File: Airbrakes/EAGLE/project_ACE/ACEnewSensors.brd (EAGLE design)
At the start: 100.3 x 62.2 mm, 21 parts, among them J3 PTH

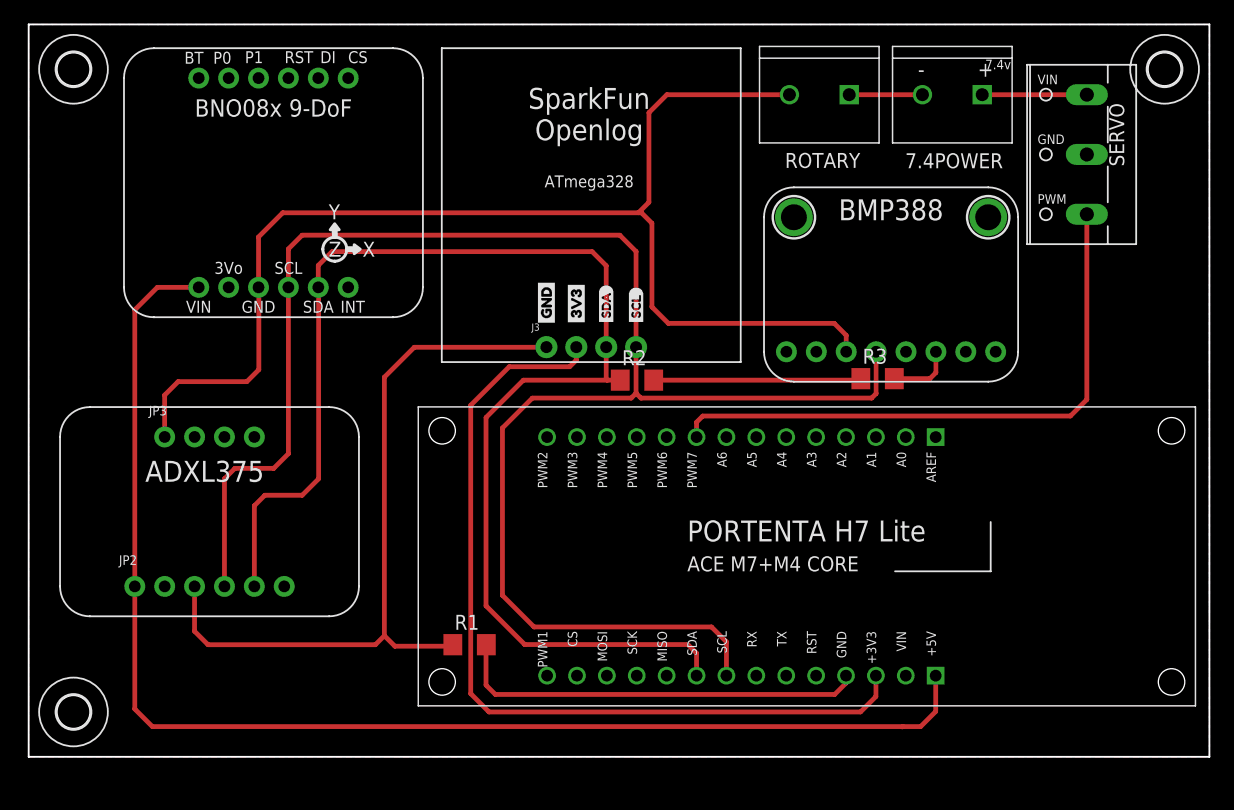
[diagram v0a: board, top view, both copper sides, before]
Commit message: Finalize v0.2 ACE PCB
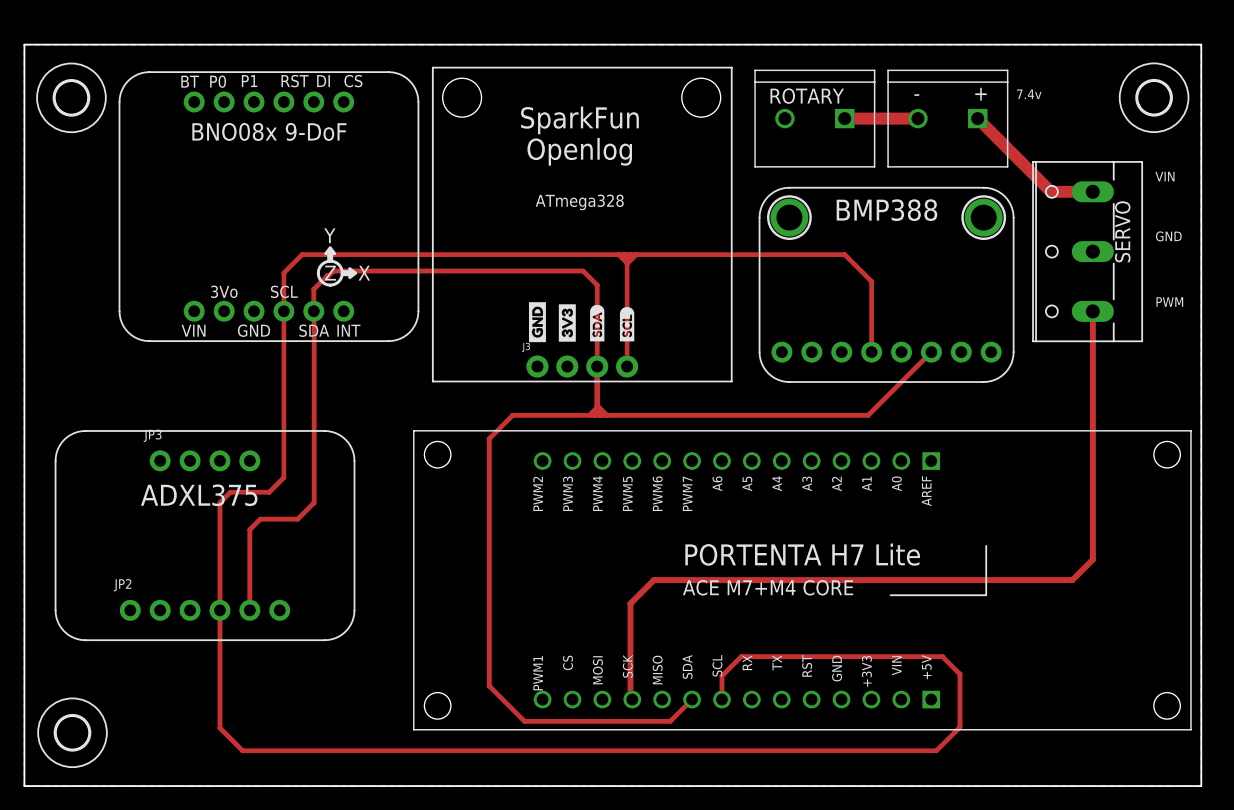
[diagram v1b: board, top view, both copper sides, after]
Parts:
- removed R1: 0 ohm, fab_new:R1206
- removed R2, R3: (no value), fab_new:R1206
- added JP4, JP5: STAND-OFF, SparkFun:STAND-OFF
- moved SERVO 8.27 mm to (112.6, 49.9)
- moved U$14 2.58 mm to (118.5, 63.0)
- moved U$13 2.44 mm to (26.5, 63.0)
- moved 7.4POWER 2.07 mm to (101.0, 61.2)
- moved ROTARY_TERMINAL 2.07 mm to (89.7, 61.2)
- moved U$5 2.07 mm to (29.3, 41.0)
- moved JP2 2.07 mm to (37.8, 19.4)
- moved JP3 2.07 mm to (37.8, 32.1)
- moved U$10 2.07 mm to (88.6, 22.0)
- moved U$8 1.82 mm to (68.6, 41.8)
- moved U$9 1.82 mm to (66.1, 41.8)
- moved J3 1.82 mm to (66.1, 40.1)
- moved U$16 1.82 mm to (71.2, 41.9)
- moved U$19 1.82 mm to (73.7, 41.9)
- moved U$15 1.77 mm to (26.6, 9.03)
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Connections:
- removed net 3.3V: J3.2, JP1.2, U$10.J17
- removed net VIN: JP1.1
- net GND: no longer R1.1
- net N$2: now also JP1.2; no longer R2.2, R3.1
- net SDA: no longer R2.1, R3.2
- net SERVO_PWM: now also U$10.J25; no longer U$10.J9
- net VCC: now also J3.2, JP1.1, U$10.J17; no longer U$10.J15
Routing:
- net GND: track 205.1 -> 0.00 mm
- net VCC: track 112.4 -> 0.00 mm
- net 3.3V: track 73.6 -> 0.00 mm
- net SCL: track 150.1 -> 205.1 mm
- net SDA: track 122.5 -> 162.0 mm
- net SERVO_PWM: track 51.0 -> 70.1 mm
- net N$2: track 17.7 -> 0.00 mm
- net SERVO_VIN: track 8.89 -> 12.4 mm
- added copper zone on layer 1, net VCC
- removed copper zone on layer 1, net GND
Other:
- board size 100.3 x 62.2 mm -> 100 x 63 mm
- board text added: "A C E"
- board text added: "AIRBRAKES COMPUTE ELEMENT"
- board text added: "May all who install this ACE onto a subscale or fullscale vehicle become the recipients of great fortune and success..."
- board text added: "v0.2 (...no more on-field soldering!)"
